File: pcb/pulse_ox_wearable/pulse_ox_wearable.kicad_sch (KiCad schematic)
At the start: 45 parts, among them J1 JST Battery In, J2 USB4800-03-A, J3 52207-0460, J4 OLED, Q1 BC817, Q2 BC817, SW1 450302014072, SW2 SW_Push, U1 ESP32-S3-WROOM-2-N32R8V, U2 MCP73832T-2DCI/OT, U3 CP2102N-Axx-xQFN24, U4 TPS61230DRC, U5 AZ1117IH-3.3TRG1

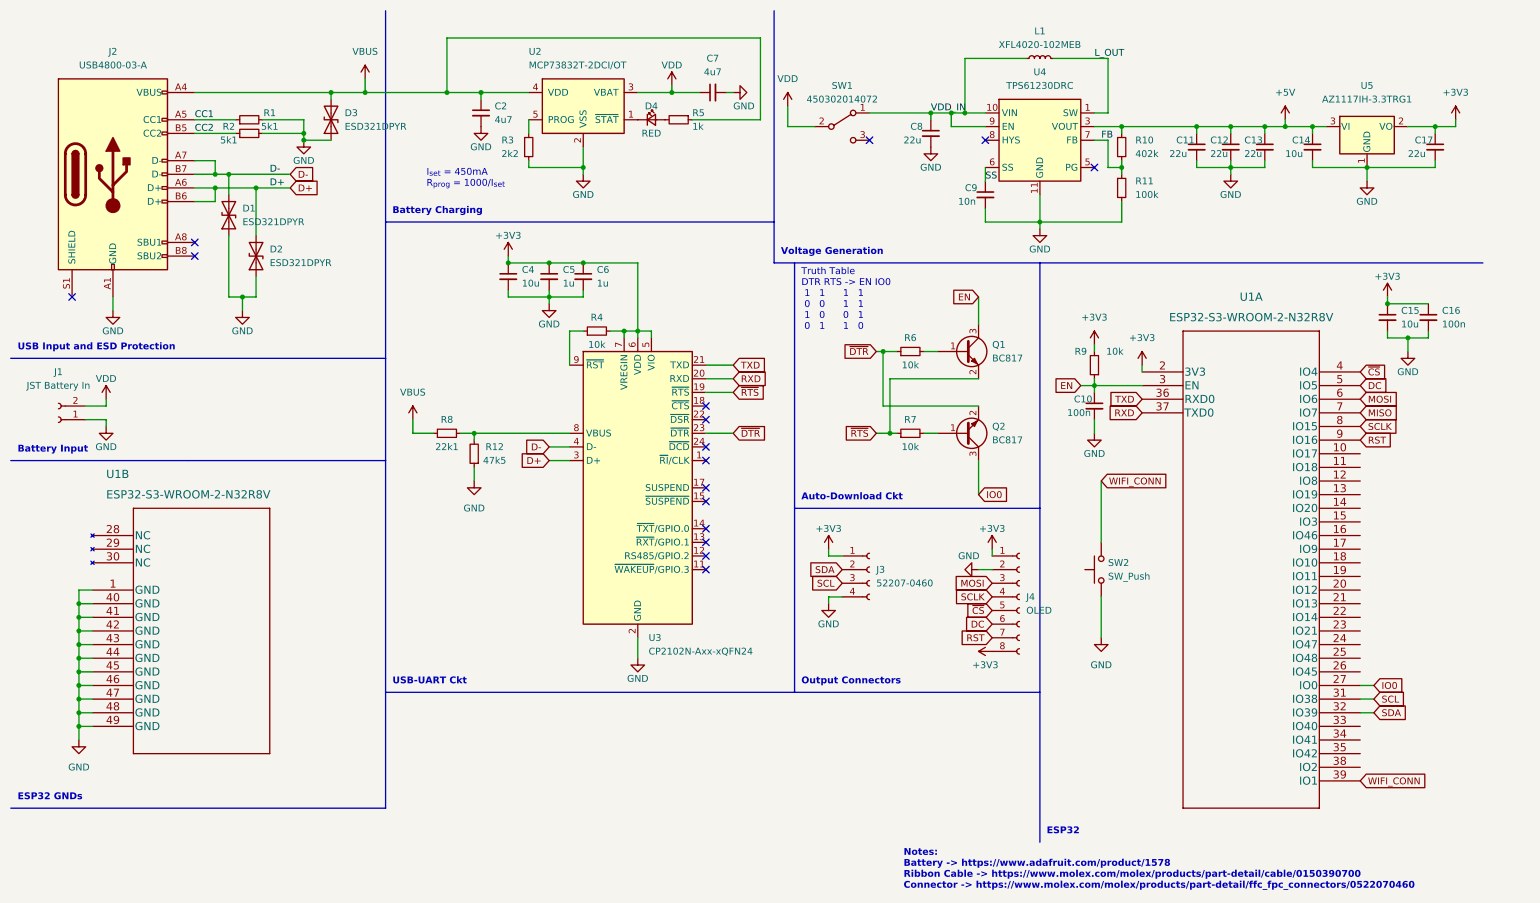
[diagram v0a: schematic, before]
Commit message: updated for week 4
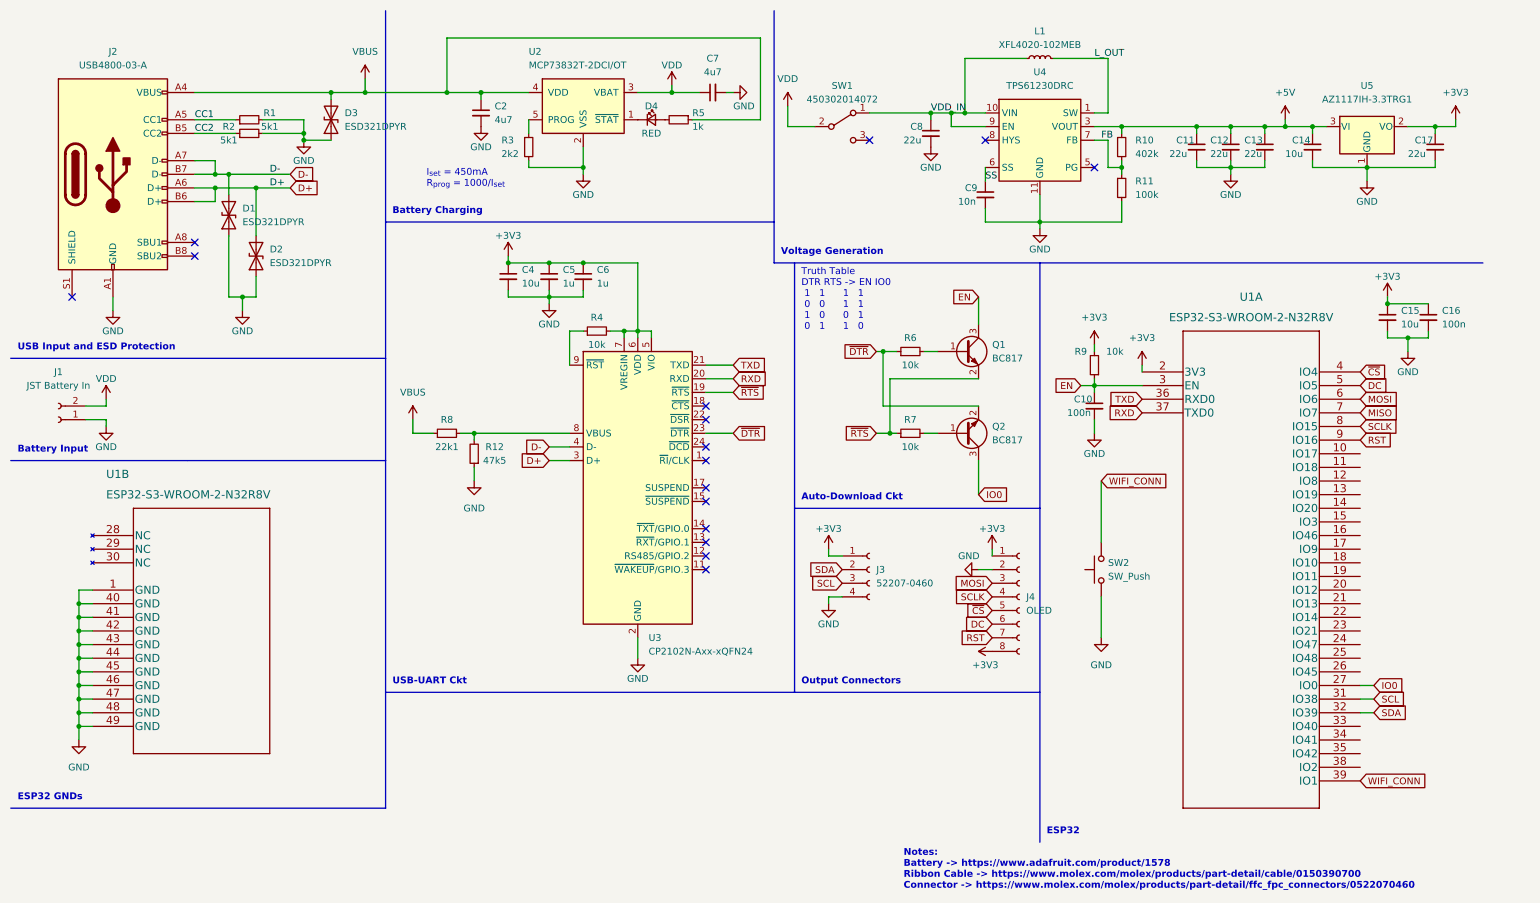
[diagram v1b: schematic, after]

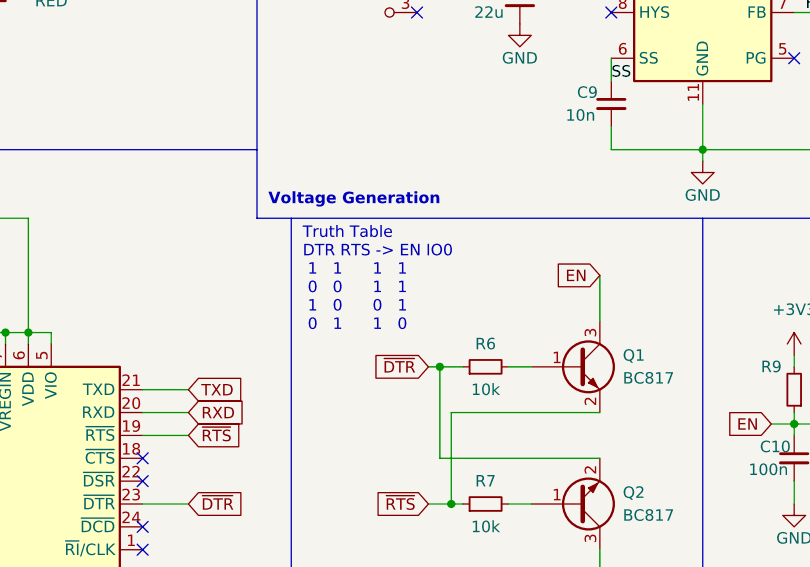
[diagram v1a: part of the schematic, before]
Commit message: uploaded code and stuff
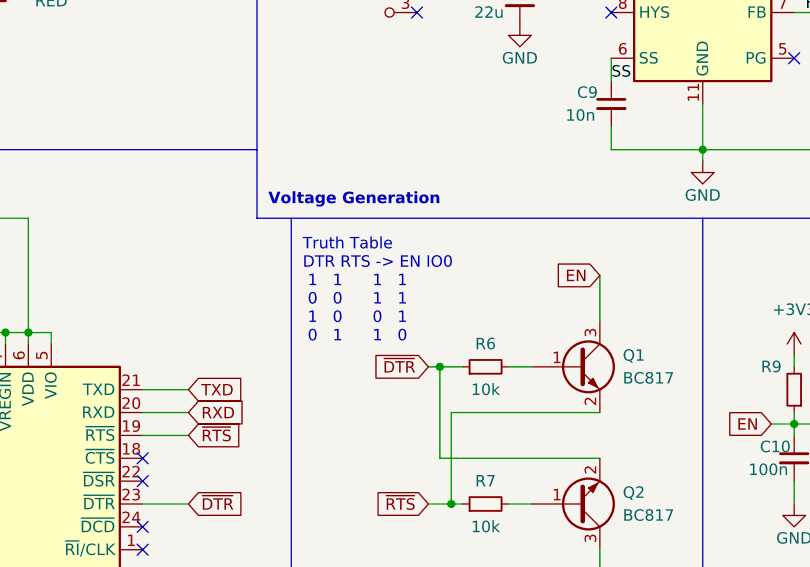
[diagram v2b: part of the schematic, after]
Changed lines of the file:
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@@
   )
   (text "Truth Table\nDTR RTS -> EN IO0\n 1   1      1   1 \n 0   0      1   1\n 1   0      0   1\n 0   1      1   0 "
-    (at 158.75 71.12 0)
+    (at 158.75 72.39 0)
     (effects (font (size 1.27 1.27)) (justify left bottom))
   )
